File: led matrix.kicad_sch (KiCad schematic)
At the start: 91 parts, among them U13 SN74LV1T125DCK

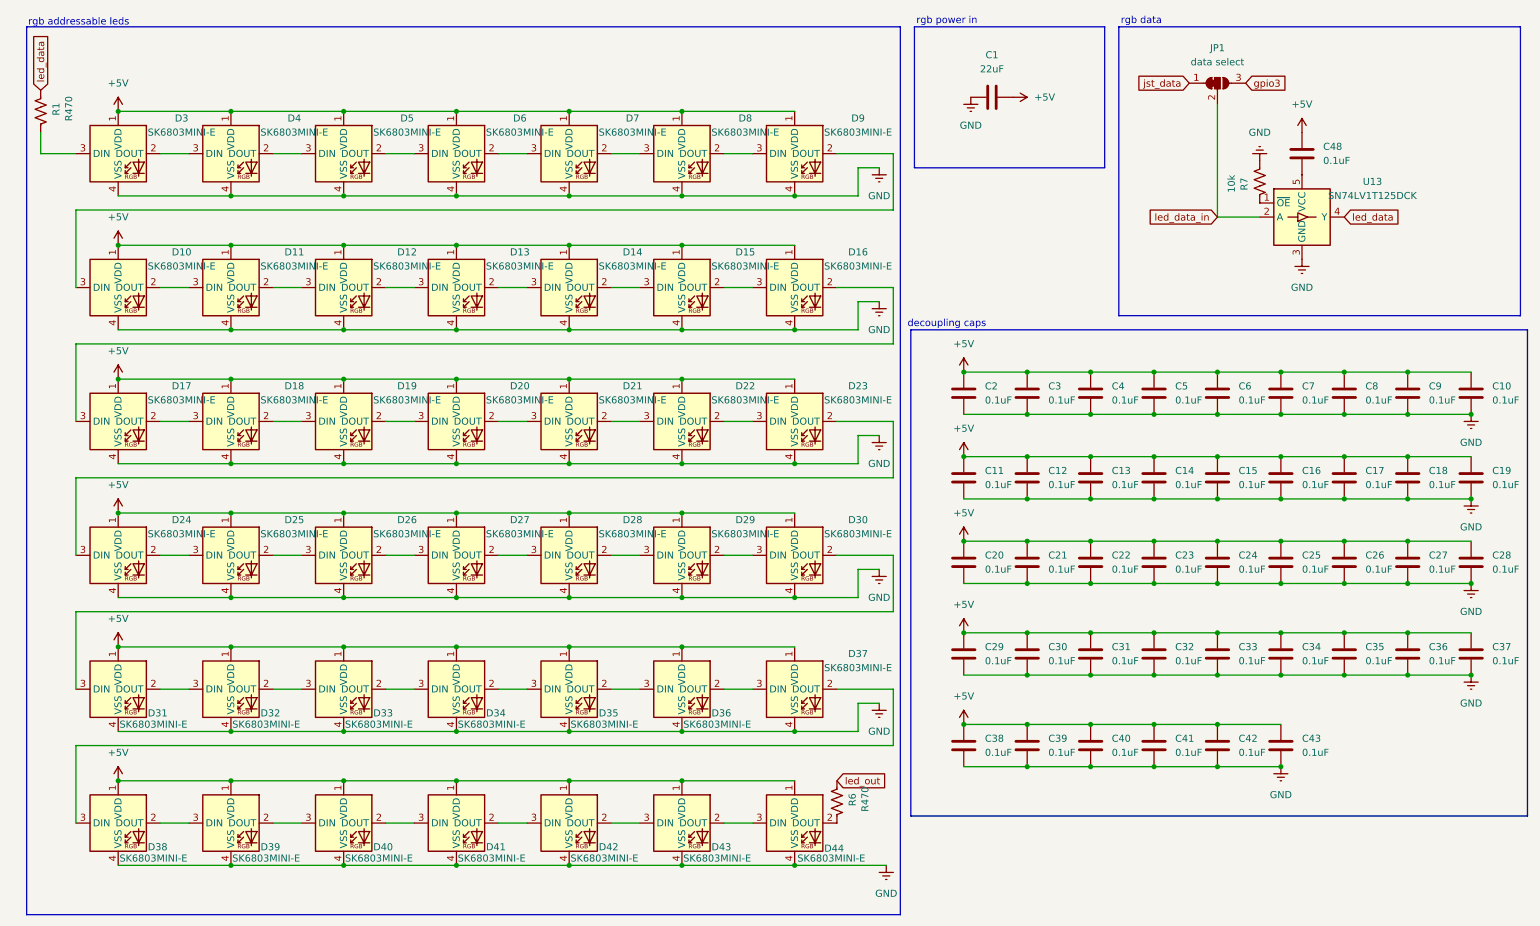
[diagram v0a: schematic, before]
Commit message: v2 final ready to order
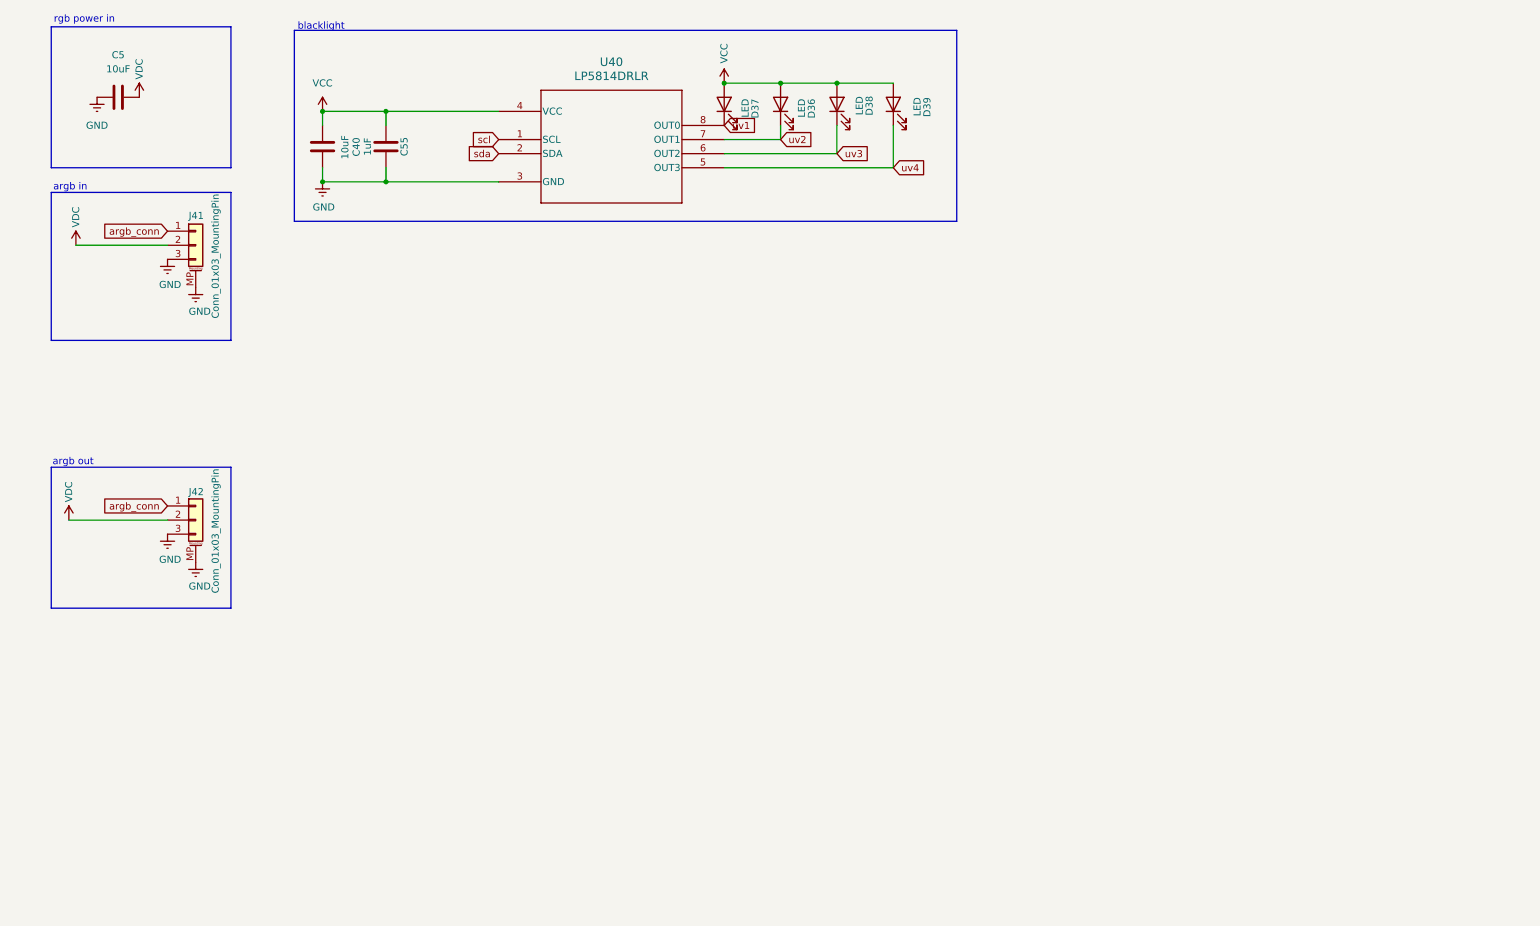
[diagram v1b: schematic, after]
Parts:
- removed C10, C11, C12, C13, C14, C15, C16, C17, C18, C19, C2, C20, C21, C22, C23, C24, C25, C26, C27, C28, C29, C3, C30, C31, C32, C33, C34, C35, C36, C37, C38, C39, C4, C41, C42, C43, C48, C5, C6, C7, C8, C9: 0.1uF, Capacitor_SMD:C_0603_1608Metric, symbol Device:C
- removed D10, D11, D12, D13, D14, D15, D16, D17, D18, D19, D20, D21, D22, D23, D24, D25, D26, D27, D28, D29, D3, D30, D31, D32, D33, D34, D35, D36, D37, D38, D39, D4, D40, D41, D42, D43, D44, D5, D6, D7, D8, D9: SK6803MINI-E, marbastlib-various:LED_6028R, symbol marbastlib-various:SK6812MINI-E
- removed JP1: data select, Jumper:SolderJumper-3_P1.3mm_Bridged12_RoundedPad1.0x1.5mm, symbol Jumper:SolderJumper_3_Bridged12
- removed R1, R6: R470, Resistor_SMD:R_0805_2012Metric, symbol Device:R_US
- removed R7: 10k, Resistor_SMD:R_0603_1608Metric, symbol Device:R_US
- removed U13: SN74LV1T125DCK, Package_TO_SOT_SMD:SOT-353_SC-70-5, symbol Logic_LevelTranslator:SN74LV1T125DCK
- added C55: 1uF, Capacitor_SMD:C_0603_1608Metric, symbol Device:C
- added D36, D37, D38, D39: LED, PCM_LED_SMD_AKL:LED_PLCC_2835, symbol Device:LED
- added J41, J42: Conn_01x03_MountingPin, Connector_JST:JST_SH_SM03B-SRSS-TB_1x03-1MP_P1.00mm_Horizontal, symbol Connector_Generic_MountingPin:Conn_01x03_MountingPin
- added U40: LP5814DRLR, Package_TO_SOT_SMD:SOT-583-8, symbol gachlilit:LP5814DRLR
- C40: value 0.1uF -> 10uF; footprint Capacitor_SMD:C_0603_1608Metric -> Capacitor_SMD:C_0805_2012Metric
- C5: renamed from C1; value 22uF -> 10uF
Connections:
- net GND: now also C55.2, J41.3 (Pin_3), J41.MP (MountPin), J42.3 (Pin_3), J42.MP (MountPin), U40.3 (GND)
- net +5V renamed VCC
- net VCC: now also C55.1, D36.2 (A), D37.2 (A), D38.2 (A), D39.2 (A), U40.4 (VCC); no longer C5.1
- new net VDC: C5.1, J41.2 (Pin_2), J42.2 (Pin_2)
- new net argb_conn: J41.1 (Pin_1), J42.1 (Pin_1)
- new net scl: U40.1 (SCL)
- new net sda: U40.2 (SDA)
- new net uv1: D37.1 (K), U40.8 (OUT0)
- new net uv2: D36.1 (K), U40.7 (OUT1)
- new net uv3: D38.1 (K), U40.6 (OUT2)
- new net uv4: D39.1 (K), U40.5 (OUT3)
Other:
- note added: "argb in"
- note added: "argb out"
- note added: "blacklight"
- note removed: "decoupling caps"
- note removed: "rgb addressable leds"
- note removed: "rgb data"
- moved on the sheet: C5
